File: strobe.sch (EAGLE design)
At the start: 50 parts, among them IC1 AT90USB162A, Q1 IRF3704S, Q2 IRF3704S, Q4 IRF3704S, Q5 IRF3704S, T1 BC849, T2 BC849, T5 BC849, T6 BC849, X6 RJ45-6LC21-B

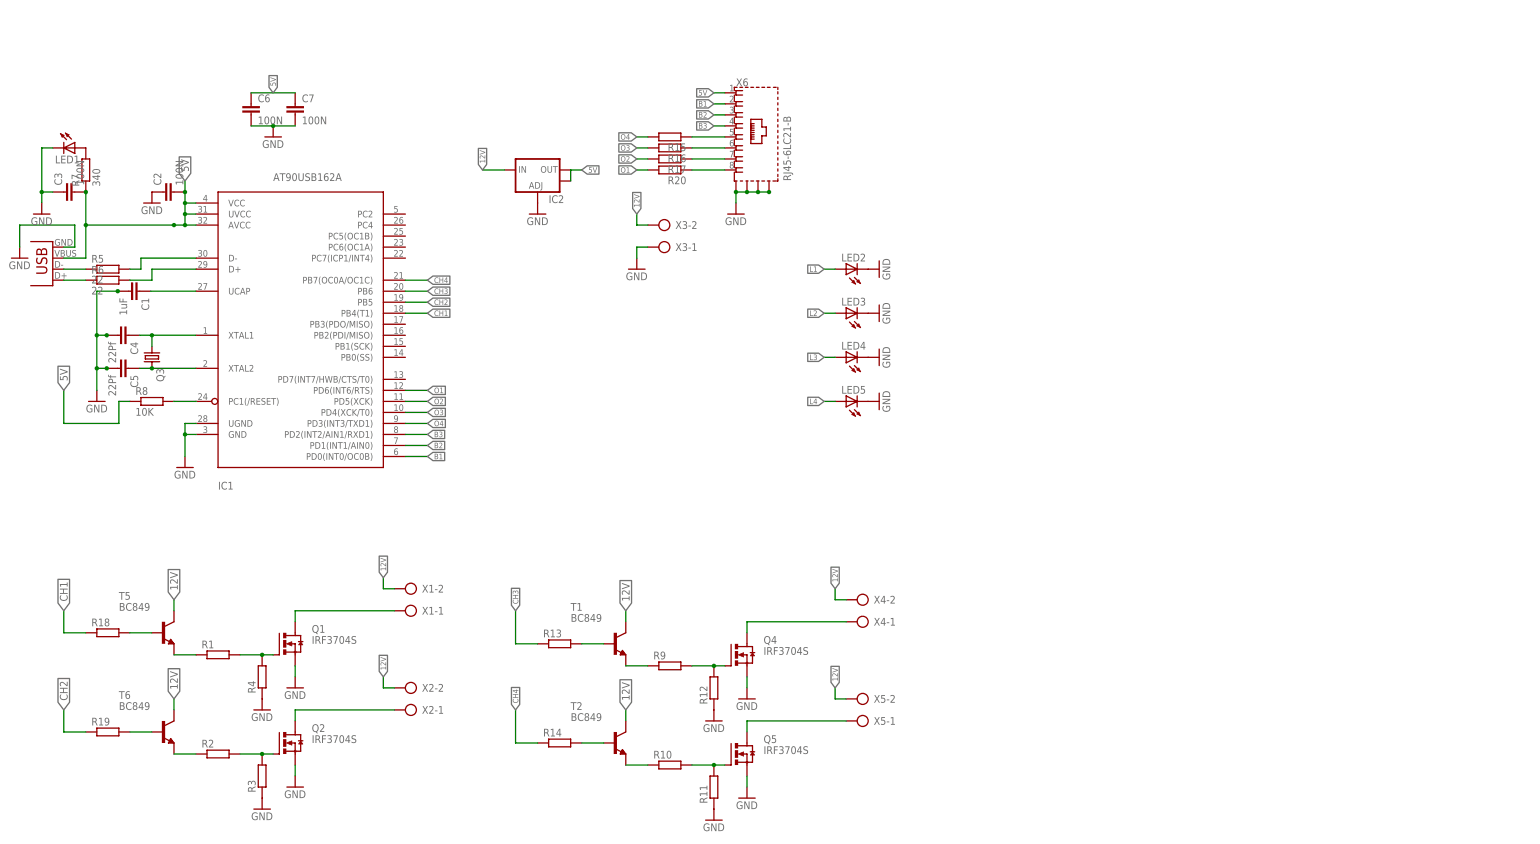
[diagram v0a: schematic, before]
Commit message: board fix
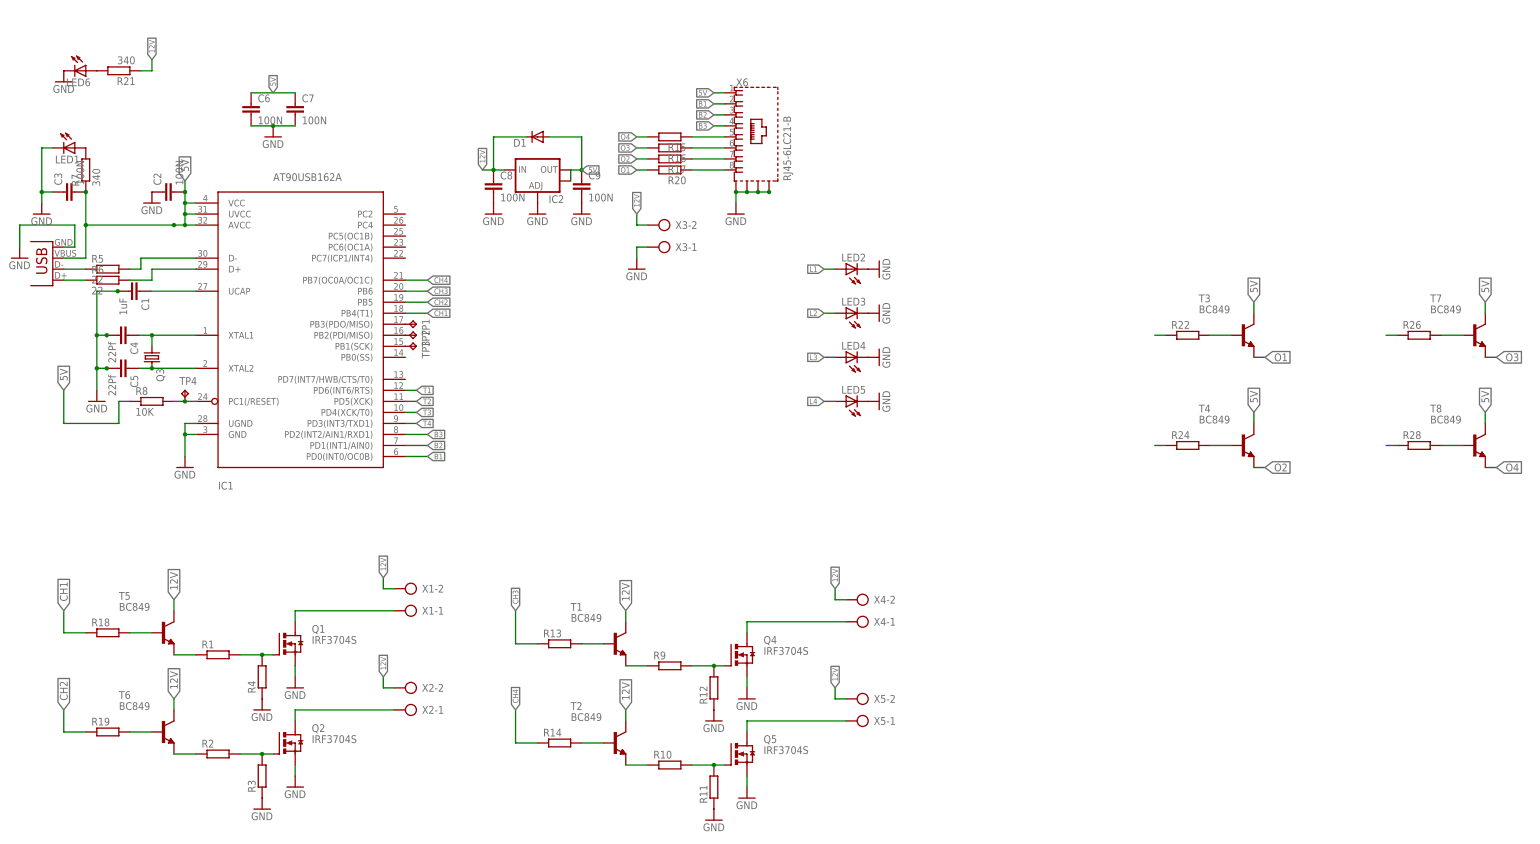
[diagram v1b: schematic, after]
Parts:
- added C8, C9: 100N, rcl:C-EUC0805
- added D1: (no value), diode:DIODE-SMB
- added LED6: (no value), led:LEDSML0805
- added R21: 340, rcl:R-EU_R0805
- added R22, R24, R26, R28: (no value), rcl:R-EU_R0805
- added T3, T4, T7, T8: BC849, transistor:BC849
- added TP1, TP2, TP3, TP4: TPB1,27, testpad:TPB1,27
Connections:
- new net N$22: IC1.PB3(PDO/MISO), TP1.TP
- new net N$23: LED6.A, R21.2
- new net N$24: R22.2, T3.B
- new net N$25: IC1.PB2(PDI/MISO), TP2.TP
- new net N$27: R24.2, T4.B
- new net N$32: IC1.PB1(SCK), TP3.TP
- new net N$34: R26.2, T7.B
- new net N$37: R28.2, T8.B
- new net T1: IC1.PD6(INT6/RTS), R22.1
- new net T2: IC1.PD5(XCK), R24.1
- new net T3: IC1.PD4(XCK/T0), R26.1
- new net T4: IC1.PD3(INT3/TXD1), R28.1
- net 12V: now also C8.1, D1.C, R21.1
- net 5V: now also C9.1, D1.A, T3.C, T4.C, T7.C, T8.C
- net GND: now also C8.2, C9.2, LED6.C
- net N$14: now also TP4.TP
- net O1: now also T3.E; no longer IC1.PD6(INT6/RTS)
- net O2: now also T4.E; no longer IC1.PD5(XCK)
- net O3: now also T7.E; no longer IC1.PD4(XCK/T0)
- net O4: now also T8.E; no longer IC1.PD3(INT3/TXD1)

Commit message: PCB extreme makeover
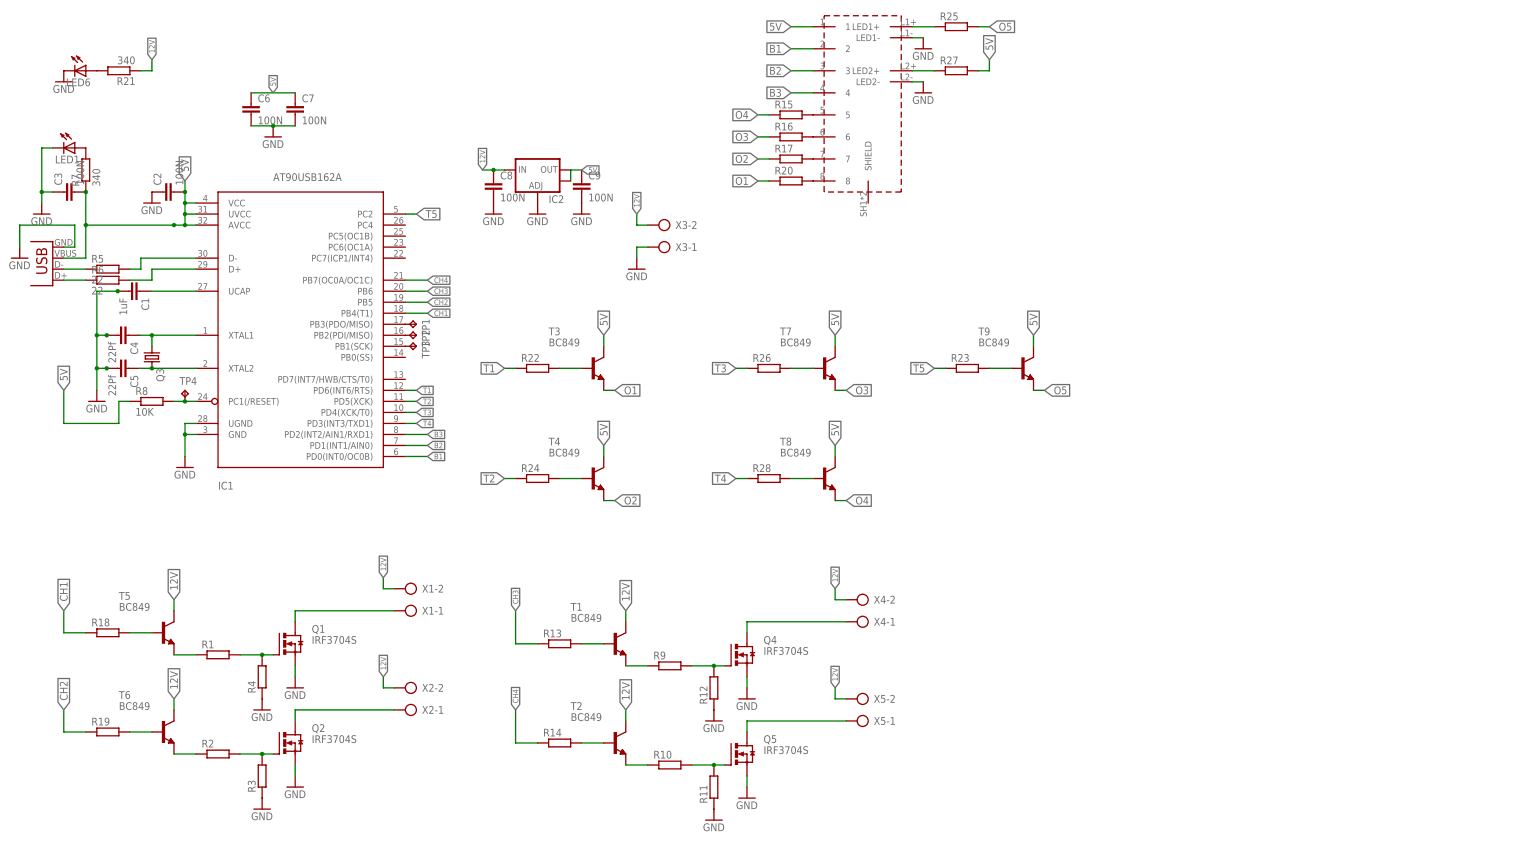
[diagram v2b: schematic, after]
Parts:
- removed D1: (no value), diode:DIODE-SMB
- removed LED2, LED3, LED4, LED5: (no value), led:LEDSML0805
- removed X6: RJ45-6LC21-B, con-tycoelectronics:RJ45-6LC21-B
- added R23, R25, R27: (no value), rcl:R-EU_R0805
- added T9: BC849, transistor:BC849
- added U$1: RJ45, RJ45:RJ45
- JP1: value USBSMD -> USB-B; device SparkFun-Connectors:USBSMD -> SparkFun-Connectors:USBPTH
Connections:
- removed net L1: LED2.A, R20.1, X6.8
- removed net L2: LED3.A, R17.1, X6.7
- removed net L3: LED4.A, R16.1, X6.6
- removed net L4: LED5.A, R15.1, X6.5
- new net N$26: R25.1, U$1.LED1+
- new net N$33: R15.2, U$1.5
- new net N$35: R16.2, U$1.6
- new net N$36: R17.2, U$1.7
- new net N$38: R20.2, U$1.8
- new net N$39: R23.2, T9.B
- new net N$40: R27.1, U$1.LED2+
- new net O5: R25.2, T9.E
- new net T5: IC1.PC2, R23.1
- net 12V: no longer D1.C
- net 5V: now also R27.2, T9.C, U$1.1; no longer D1.A, X6.1
- net B1: now also U$1.2; no longer X6.2
- net B2: now also U$1.3; no longer X6.3
- net B3: now also U$1.4; no longer X6.4
- net GND: now also U$1.LED1-, U$1.LED2-; no longer LED2.C, LED3.C, LED4.C, LED5.C, X6.S@1, X6.S@2, X6.S@3, X6.S@4
- net O1: now also R20.1; no longer R20.2
- net O2: now also R17.1; no longer R17.2
- net O3: now also R16.1; no longer R16.2
- net O4: now also R15.1; no longer R15.2
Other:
- moved on the sheet: R15, R16, R17, R20, R22, R24, R26, R28, T3, T4, T7, T8
